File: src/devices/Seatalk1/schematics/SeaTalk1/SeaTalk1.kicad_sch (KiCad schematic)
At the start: 30 parts, among them J1 Raspberry_Pi_2_3, J3 Conn_01x03_Pin, Q1 BC557, Q2 BC547, Q3 BC547, Q4 BC547, Q5 BC547, Q6 BC547

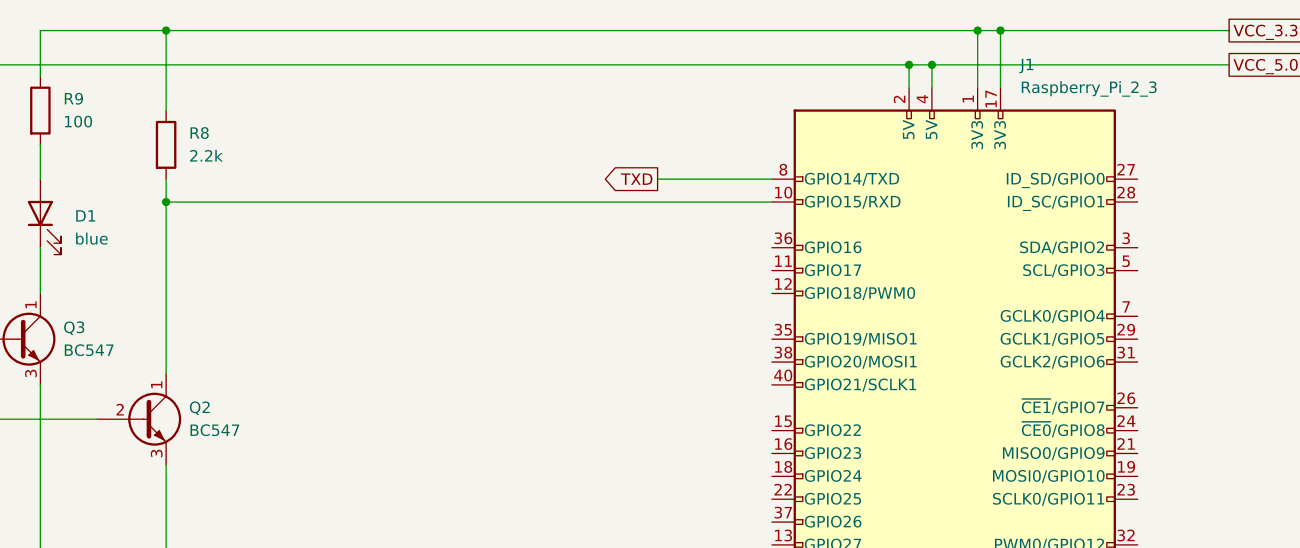
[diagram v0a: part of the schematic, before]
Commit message: Documentation started
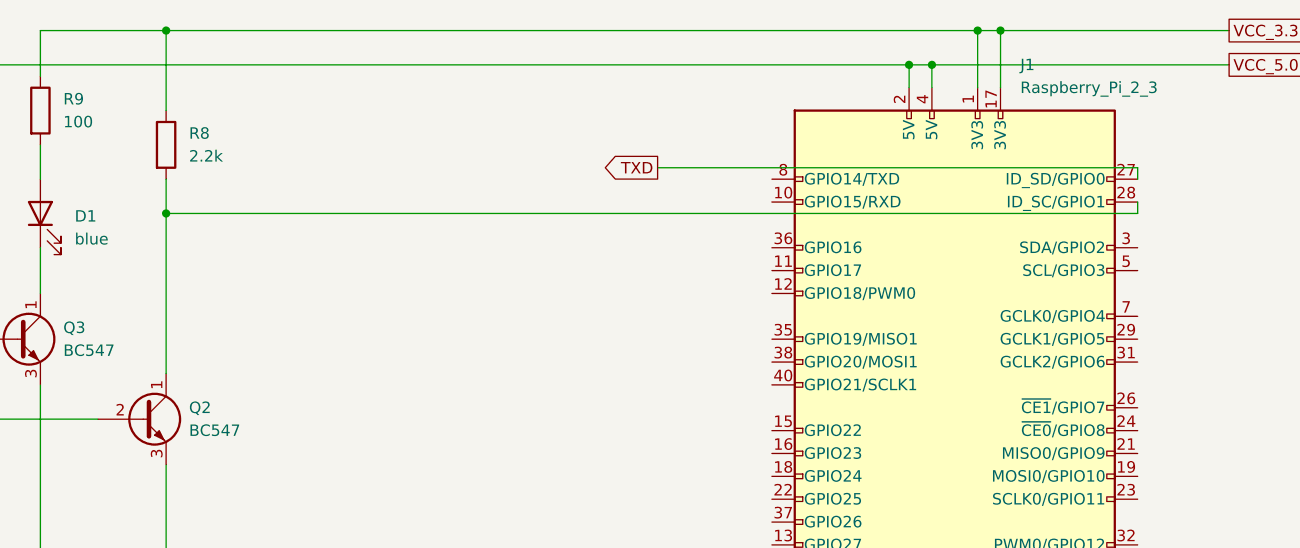
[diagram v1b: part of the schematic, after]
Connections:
- net TXD: now also J1.27 (ID_SD/GPIO0); no longer J1.8 (GPIO14/TXD)
- net at Q2.1 (C), R8.2: now also J1.28 (ID_SC/GPIO1); no longer J1.10 (GPIO15/RXD)
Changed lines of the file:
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@@
   (junction (at 236.22 161.29) (diameter 0) (color 0 0 0 0)
   )
-  (junction (at 148.59 38.1) (diameter 0) (color 0 0 0 0)
-  )
   (junction (at 241.3 19.05) (diameter 0) (color 0 0 0 0)
   )
@@
   (junction (at 93.98 71.12) (diameter 0) (color 0 0 0 0)
   )
+  (junction (at 148.59 39.37) (diameter 0) (color 0 0 0 0)
+  )
   (junction (at 231.14 22.86) (diameter 0) (color 0 0 0 0)
   )
@@
     (stroke (width 0) (type default))
   )
+  (wire (pts (xy 203.2 34.29) (xy 256.54 34.29))
+    (stroke (width 0) (type default))
+  )
   (wire (pts (xy 224.79 161.29) (xy 236.22 161.29))
     (stroke (width 0) (type default))
@@
     (stroke (width 0) (type default))
   )
-  (wire (pts (xy 203.2 35.56) (xy 215.9 35.56))
-    (stroke (width 0) (type default))
-  )
   (wire (pts (xy 71.12 69.85) (xy 71.12 67.31))
     (stroke (width 0) (type default))
@@
     (stroke (width 0) (type default))
   )
+  (wire (pts (xy 256.54 34.29) (xy 256.54 35.56))
+    (stroke (width 0) (type default))
+  )
   (wire (pts (xy 148.59 160.02) (xy 167.64 160.02))
     (stroke (width 0) (type default))
@@
     (stroke (width 0) (type default))
   )
+  (wire (pts (xy 148.59 39.37) (xy 148.59 57.15))
+    (stroke (width 0) (type default))
+  )
   (wire (pts (xy 71.12 53.34) (xy 77.47 53.34))
     (stroke (width 0) (type default))
   )
-  (wire (pts (xy 148.59 35.56) (xy 148.59 38.1))
+  (wire (pts (xy 148.59 35.56) (xy 148.59 39.37))
     (stroke (width 0) (type default))
   )
@@
     (stroke (width 0) (type default))
   )
-  (wire (pts (xy 148.59 38.1) (xy 148.59 57.15))
-    (stroke (width 0) (type default))
-  )
   (wire (pts (xy 134.62 91.44) (xy 148.59 91.44))
     (stroke (width 0) (type default))
@@
     (stroke (width 0) (type default))
   )
+  (wire (pts (xy 148.59 39.37) (xy 256.54 39.37))
+    (stroke (width 0) (type default))
+  )
   (wire (pts (xy 168.91 115.57) (xy 168.91 119.38))
     (stroke (width 0) (type default))
@@
     (stroke (width 0) (type default))
   )
+  (wire (pts (xy 256.54 38.1) (xy 256.54 39.37))
+    (stroke (width 0) (type default))
+  )
   (wire (pts (xy 148.59 19.05) (xy 148.59 27.94))
     (stroke (width 0) (type default))
@@
   )
   (wire (pts (xy 148.59 100.33) (xy 168.91 100.33))
-    (stroke (width 0) (type default))
-  )
-  (wire (pts (xy 148.59 38.1) (xy 215.9 38.1))
     (stroke (width 0) (type default))
   )
@@
     )
   )
-  (global_label "TXD" (shape output) (at 203.2 35.56 180) (fields_autoplaced)
+  (global_label "TXD" (shape output) (at 203.2 34.29 180) (fields_autoplaced)
     (effects (font (size 1.27 1.27)) (justify right))
-    (property "Intersheetrefs" "${INTERSHEET_REFS}" (at 196.7677 35.56 0)
+    (property "Intersheetrefs" "${INTERSHEET_REFS}" (at 196.7677 34.29 0)
       (effects (font (size 1.27 1.27)) (justify right) hide)
     )
